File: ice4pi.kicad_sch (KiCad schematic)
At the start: 25 parts, among them J1 Conn_02x03, J2 Raspberry_Pi_2_3, J3 USB_C_Receptacle_USB2.0, J4 RJ45_Amphenol_RJMG1BD3B8K1ANR, U1 ENC28J60x-SS, U2 DSC1001DE1-025.0000

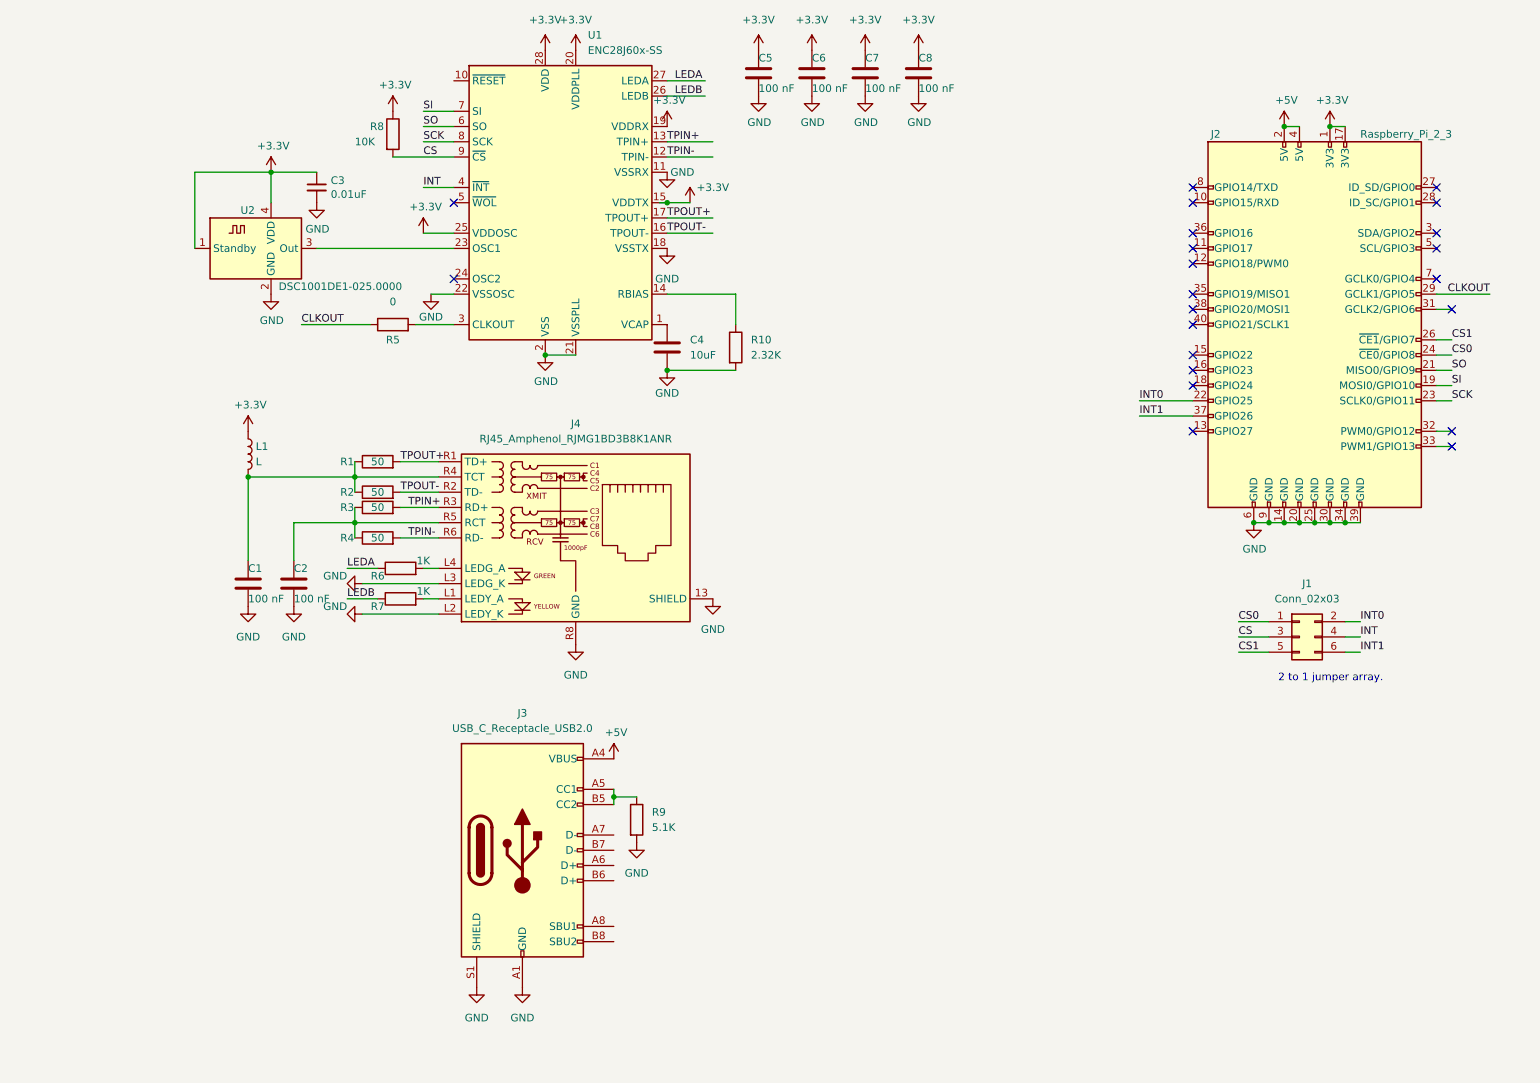
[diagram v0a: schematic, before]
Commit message: feat: poe
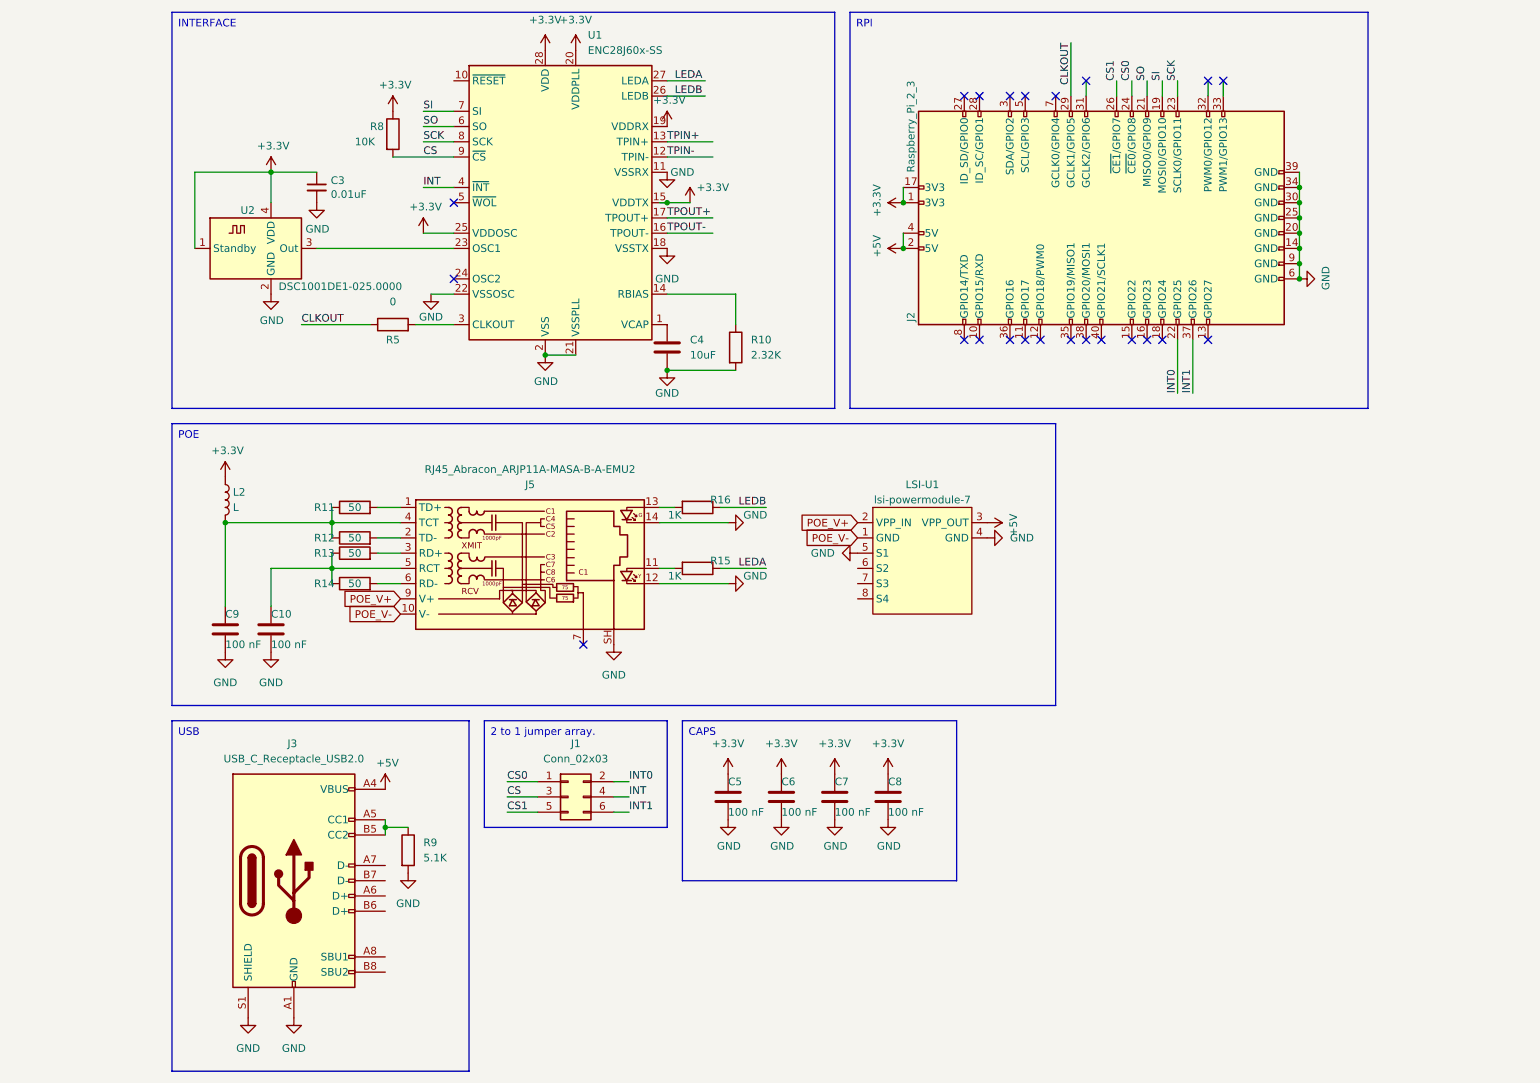
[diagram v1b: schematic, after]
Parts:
- removed C1, C2: 100 nF, Capacitor_SMD:C_0402_1005Metric, symbol Device:C
- removed J4: RJ45_Amphenol_RJMG1BD3B8K1ANR, Connector_RJ:RJ45_Amphenol_RJMG1BD3B8K1ANR, symbol Connector:RJ45_Amphenol_RJMG1BD3B8K1ANR
- removed L1: L, Inductor_SMD:L_1210_3225Metric, symbol Device:L
- removed R1, R2, R3, R4: 50, Resistor_SMD:R_0402_1005Metric, symbol Device:R
- removed R6, R7: 1K, Resistor_SMD:R_0402_1005Metric, symbol Device:R
- added C10, C9: 100 nF, Capacitor_SMD:C_0402_1005Metric, symbol Device:C
- added J5: RJ45_Abracon_ARJP11A-MASA-B-A-EMU2, Connector_RJ:RJ45_Abracon_ARJP11A-MA_Horizontal, symbol Connector:RJ45_Abracon_ARJP11A-MASA-B-A-EMU2
- added L2: L, Inductor_SMD:L_1210_3225Metric, symbol Device:L
- added LSI-U1: lsi-powermodule-7, lsi:lsi-powermodule-7, symbol lsi:lsi-powermodule-7
- added R11, R12, R13, R14: 50, Resistor_SMD:R_0402_1005Metric, symbol Device:R
- added R15, R16: 1K, Resistor_SMD:R_0402_1005Metric, symbol Device:R
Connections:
- net +3.3V: now also L2.1
- net +5V: now also LSI-U1.3 (VPP_OUT)
- net GND: now also C10.2, C9.2, J5.12, J5.14, J5.SH, LSI-U1.4 (GND), LSI-U1.5 (S1)
- net LEDA: now also R15.1
- net LEDB: now also R16.1
- new net: C9.1, J5.4 (TCT), L2.2, R11.1, R12.1
- new net: C10.1, J5.5 (RCT), R13.1, R14.1
- new net: J5.6 (RD-), R14.2
- new net: J5.3 (RD+), R13.2
- new net: J5.1 (TD+), R11.2
- new net: J5.11, R15.2
- new net: J5.13, R16.2
- new net: J5.2 (TD-), R12.2
- new net POE_V+: J5.9 (V+), LSI-U1.2 (VPP_IN)
- new net POE_V-: J5.10 (V-), LSI-U1.1 (GND)
- no-connect marks 22 -> 23
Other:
- note removed: "2 to 1 jumper array."
- moved on the sheet: C5, C6, C7, C8, J1, J2, J3, R9

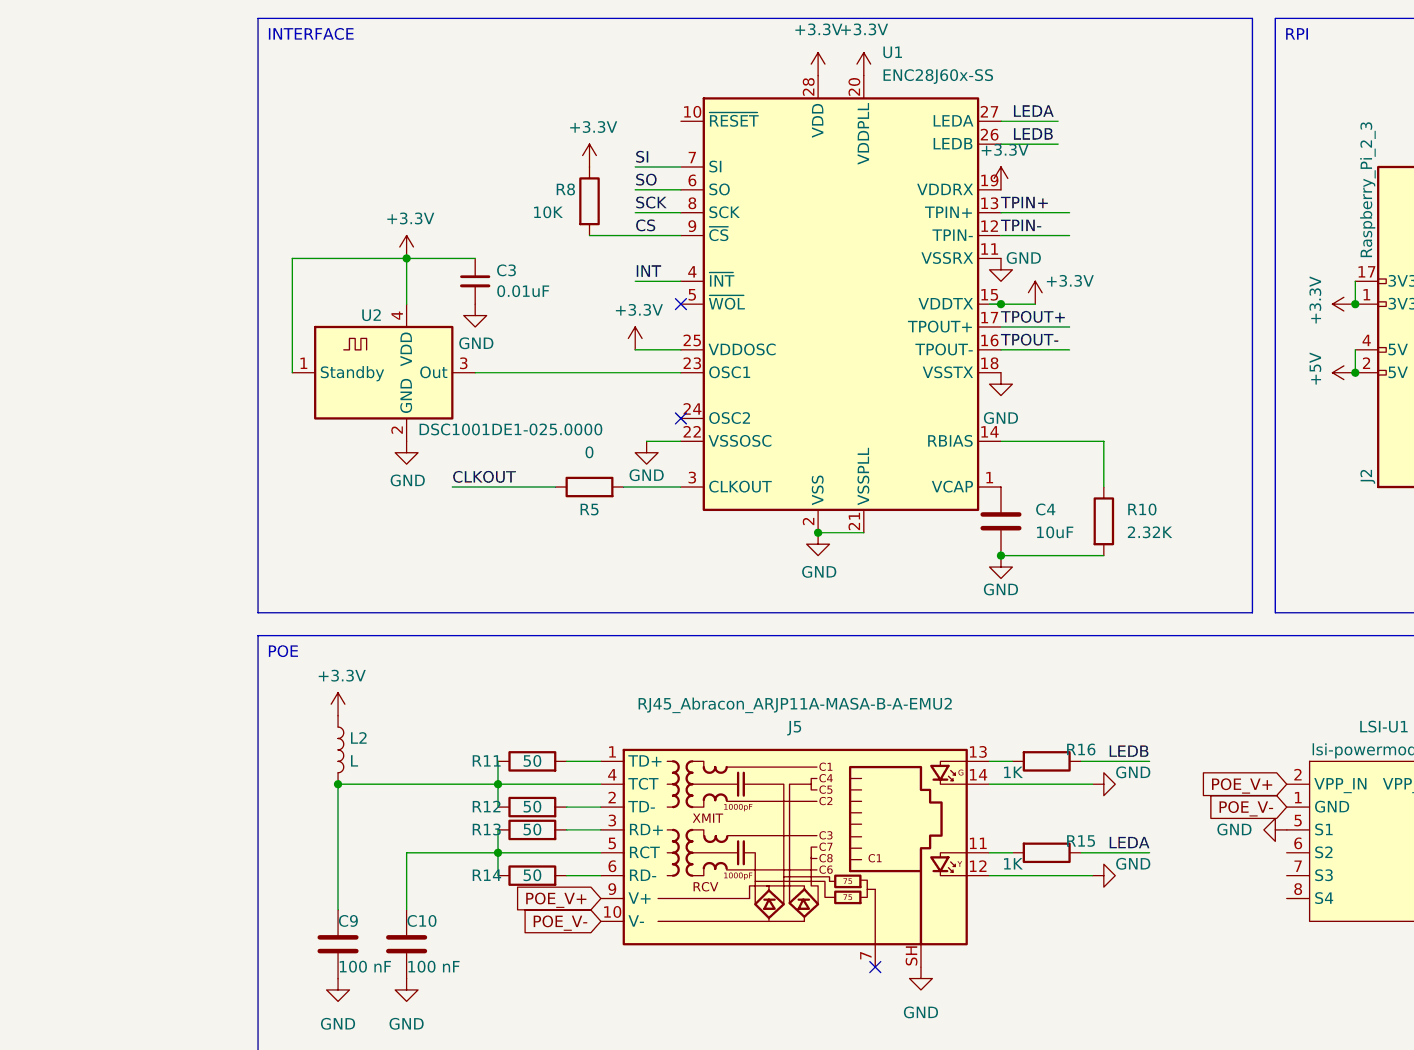
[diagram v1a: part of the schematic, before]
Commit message: feat: commit 2
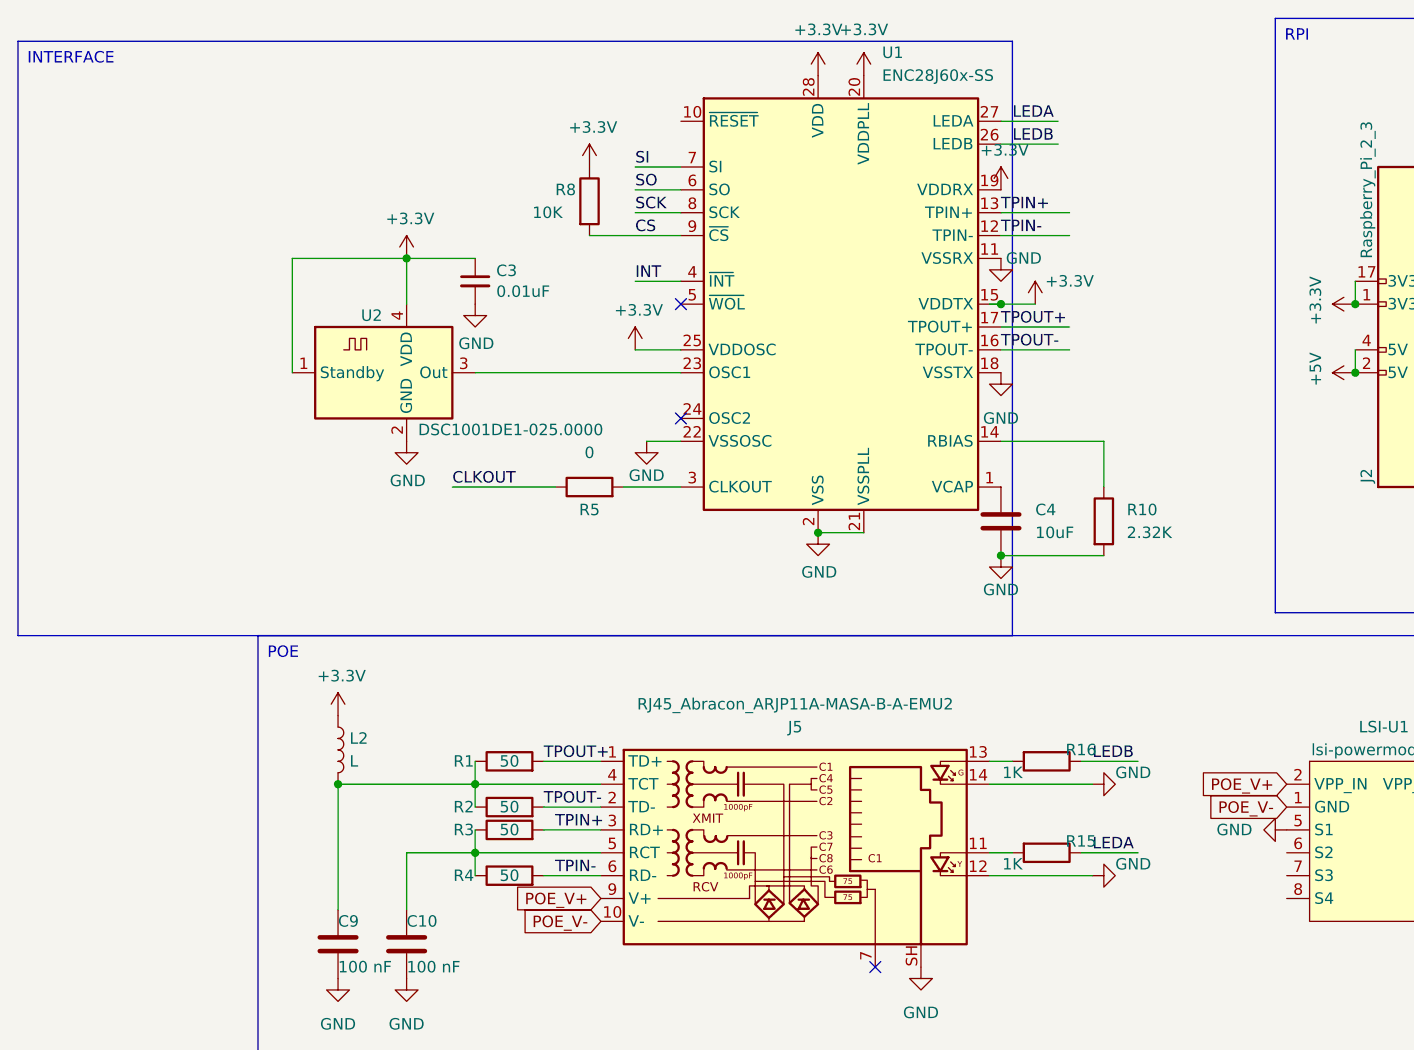
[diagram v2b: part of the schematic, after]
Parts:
- removed R11, R12, R13, R14: 50, Resistor_SMD:R_0402_1005Metric, symbol Device:R
- added R1, R2, R3, R4: 50, Resistor_SMD:R_0402_1005Metric, symbol Device:R
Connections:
- net TPIN+: now also J5.3 (RD+), R3.2
- net TPIN-: now also J5.6 (RD-), R4.2
- net TPOUT+: now also J5.1 (TD+), R1.2
- net TPOUT-: now also J5.2 (TD-), R2.2
- net at C9.1, J5.4 (TCT), L2.2: now also R1.1, R2.1
- net at C10.1, J5.5 (RCT): now also R3.1, R4.1

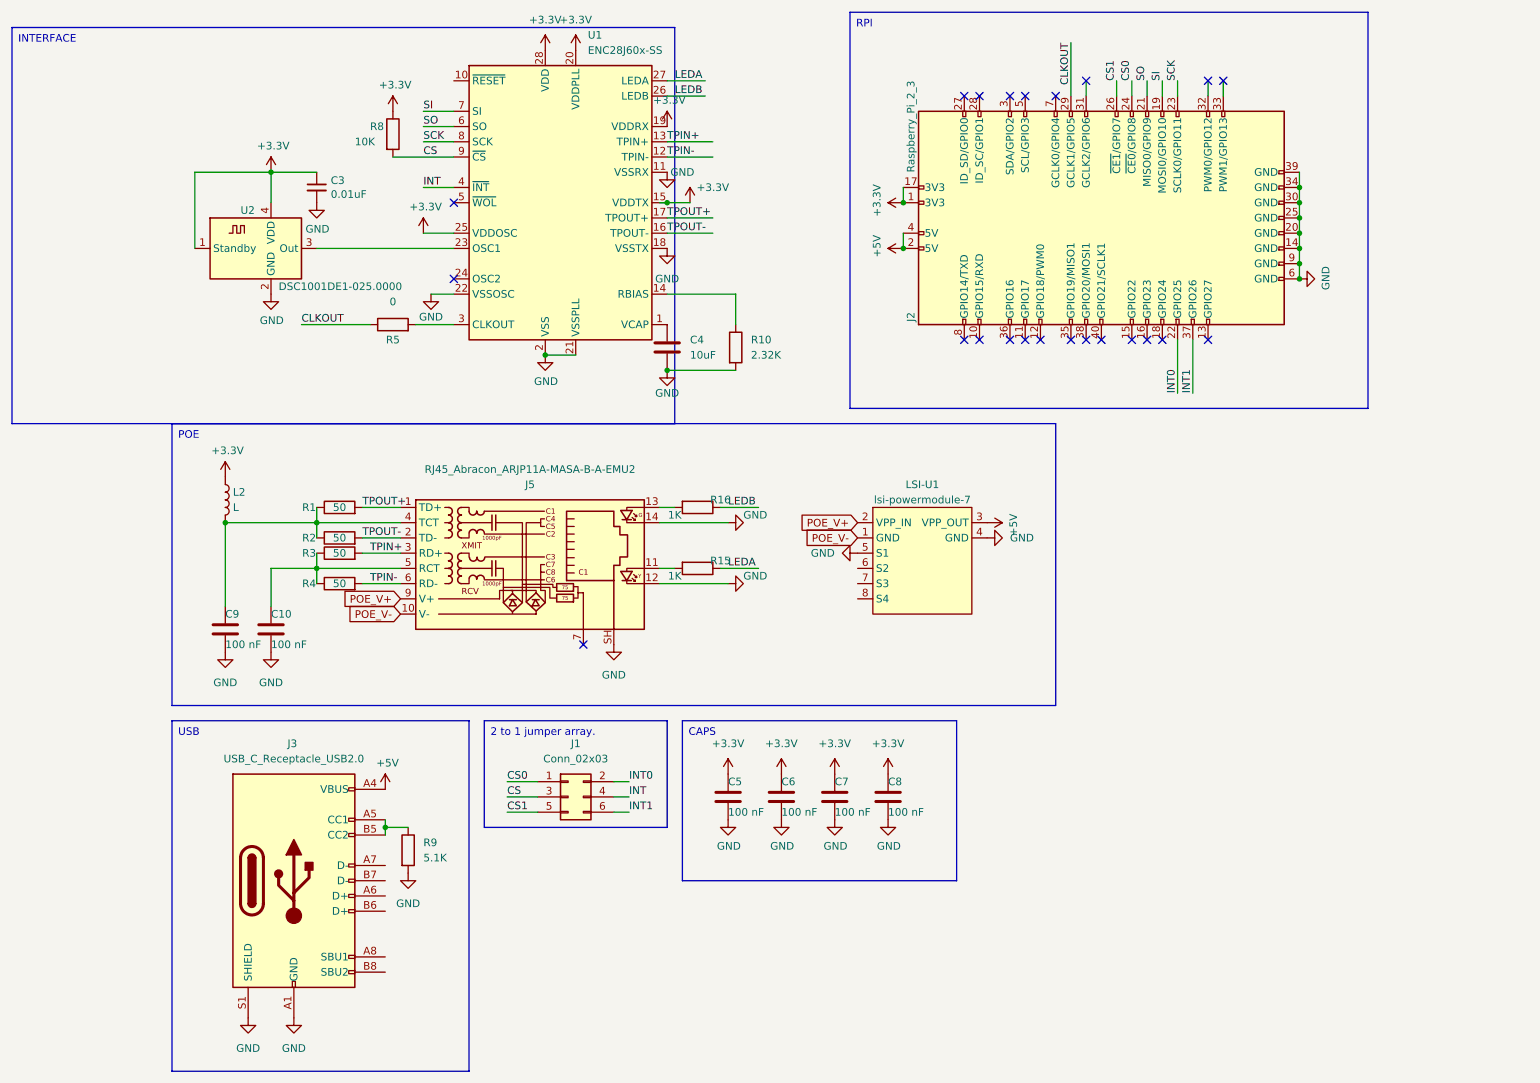
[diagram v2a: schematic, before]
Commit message: feat: poe controller
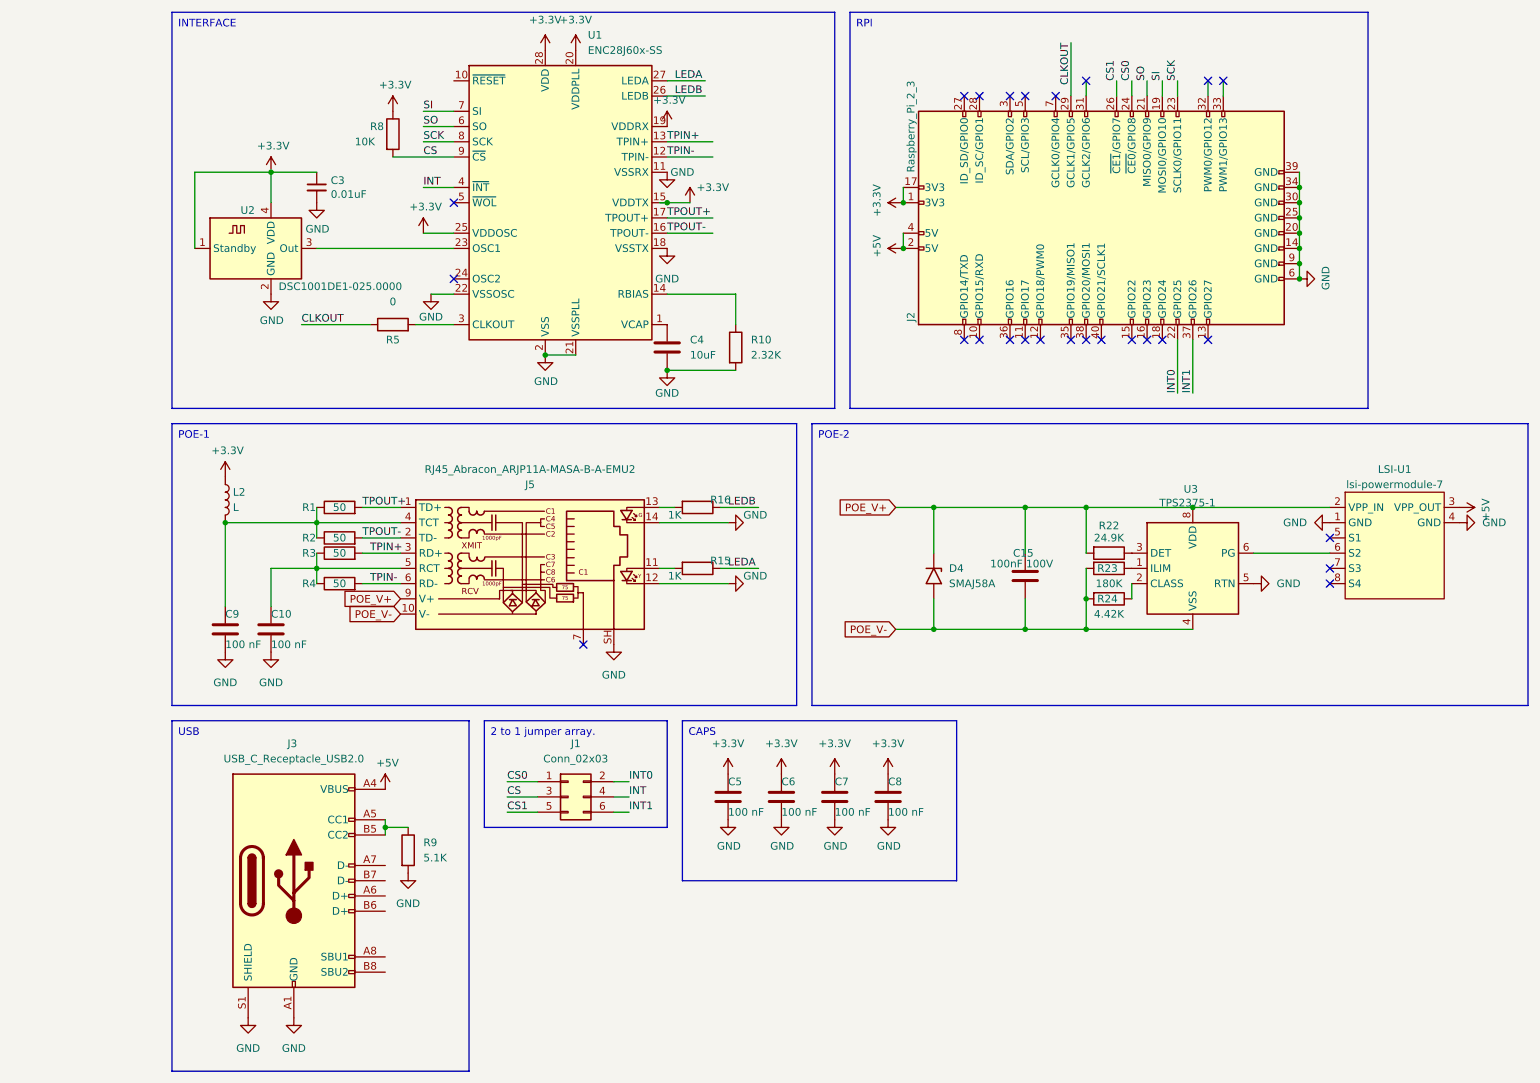
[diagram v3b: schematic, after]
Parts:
- added C15: 100nF 100V, Capacitor_SMD:C_01005_0402Metric, symbol Device:C
- added D4: SMAJ58A, Diode_SMD:D_SMA, symbol Diode:SMAJ58A
- added R22: 24.9K, Resistor_SMD:R_0402_1005Metric, symbol Device:R
- added R23: 180K, Resistor_SMD:R_0402_1005Metric, symbol Device:R
- added R24: 4.42K, Resistor_SMD:R_0402_1005Metric, symbol Device:R
- added U3: TPS2375-1, Package_SO:TSSOP-8_4.4x3mm_P0.65mm, symbol Regulator_Controller:TPS2375-1
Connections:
- net GND: now also LSI-U1.1 (GND), U3.5 (RTN); no longer LSI-U1.5 (S1)
- net POE_V+: now also C15.1, D4.1 (A1), R22.2, U3.8 (VDD)
- net POE_V-: now also C15.2, D4.2 (A2), R23.2, R24.2, U3.4 (VSS); no longer LSI-U1.1 (GND)
- net at LSI-U1.6 (S2): now also U3.6 (PG)
- new net: R22.1, U3.3 (DET)
- new net: R24.1, U3.2 (CLASS)
- new net: R23.1, U3.1 (ILIM)
- no-connect marks 23 -> 26
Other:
- title: ethernet4pizero-1.0 -> ethernet4pizero-poe-1.0
- moved on the sheet: LSI-U1
